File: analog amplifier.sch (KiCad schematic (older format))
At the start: 9 parts, among them U1 AD812

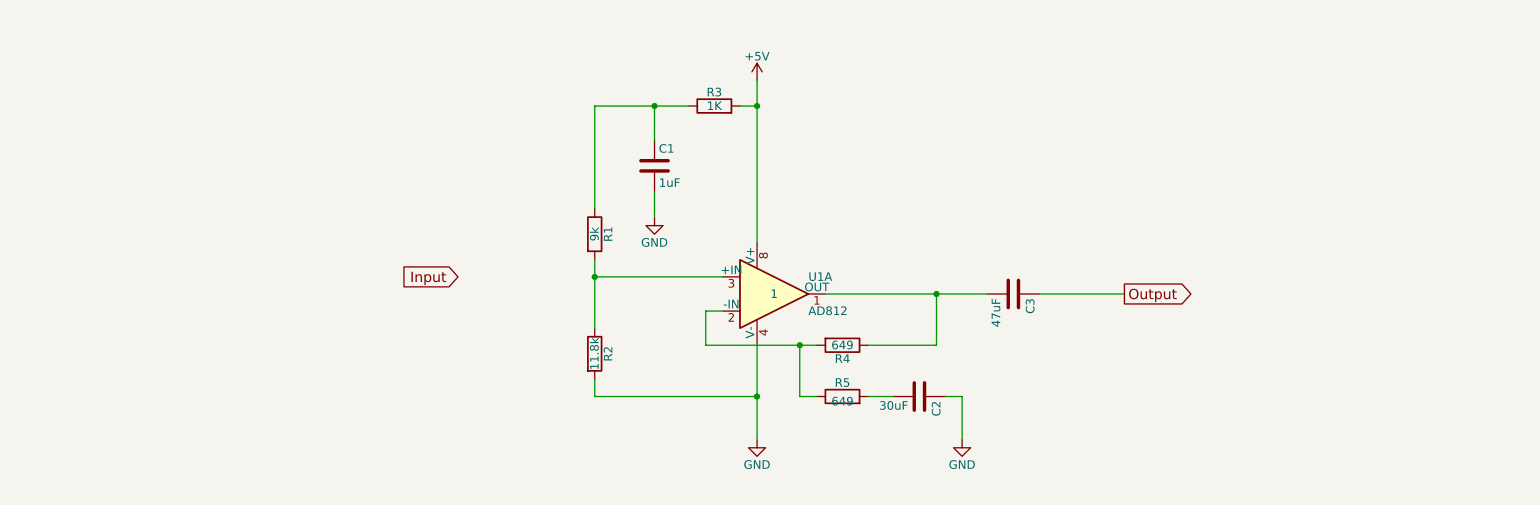
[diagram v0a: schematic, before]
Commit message: Add files via upload
Schematics and BOM
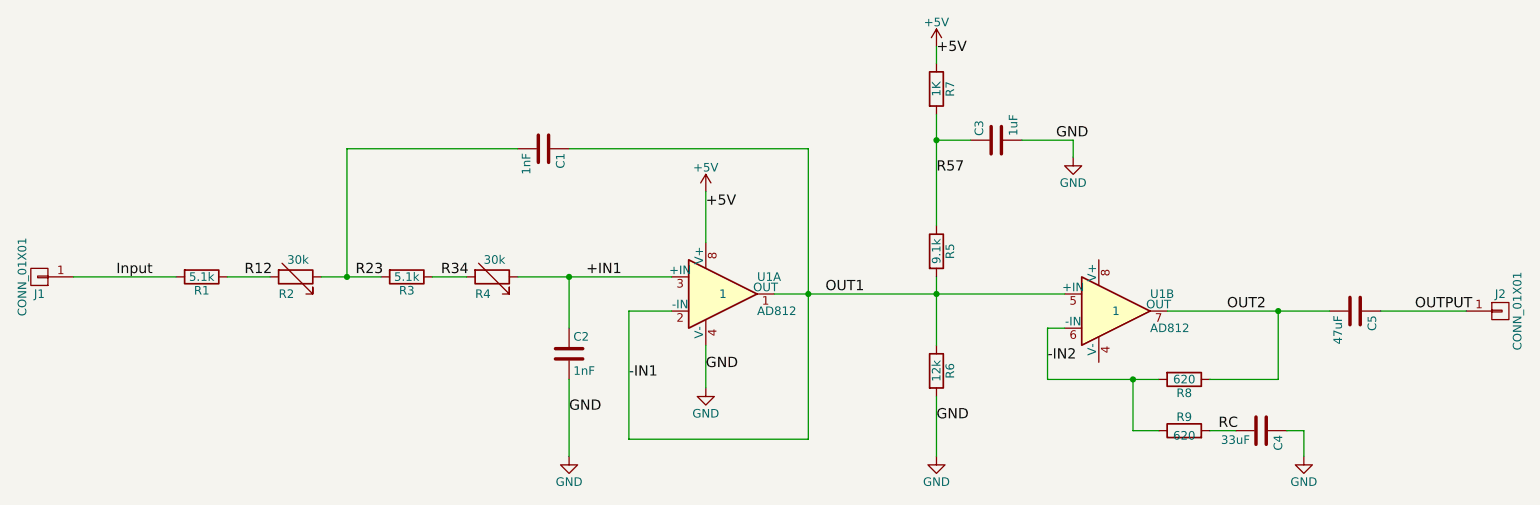
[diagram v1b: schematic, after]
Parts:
- added C1, C2: 1nF, Capacitors_SMD:C_0402, symbol C
- added J1, J2: CONN_01X01, Connectors:Banana_Jack_1Pin, symbol CONN_01X01
- added R1, R3: 5.1k, Resistors_SMD:R_0402, symbol R
- added R2, R4: 30k, Resistors_SMD:R_2816, symbol R_Variable
- added unit 1 of U1
- C3: renamed from C1; footprint (none) -> Capacitors_SMD:C_0603
- C4: renamed from C2; value 30uF -> 33uF; footprint (none) -> Capacitors_SMD:C_0805
- C5: renamed from C3; footprint (none) -> Capacitors_SMD:C_0805
- R5: renamed from R1; value 9k -> 9.1k; footprint (none) -> Resistors_SMD:R_0402
- R6: renamed from R2; value 11.8k -> 12k; footprint (none) -> Resistors_SMD:R_0402
- R7: renamed from R3; footprint (none) -> Resistors_SMD:R_0402
- R8: renamed from R4; value 649 -> 620; footprint (none) -> Resistors_SMD:R_0402
- R9: renamed from R5; value 649 -> 620; footprint (none) -> Resistors_SMD:R_0402
- U1: footprint (none) -> SMD_Packages:SOIC-8-N
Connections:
- net +5V: now also R7.1, U1.8 (V+); no longer R7.2, U1.8 (V+)
- net GND: now also C2.2, U1.4 (V-); no longer U1.4 (V-)
- net Input: now also J1.1 (P1), R1.2
- net OUT2: now reaches C5.2, R8.1
- net OUT2: now also U1.7 (OUT); no longer U1.1 (OUT)
- net -IN2: now reaches R8.2, R9.1
- net -IN2: now also U1.6 (-IN); no longer U1.2 (-IN)
- net -IN1: now reaches R5.2, R6.1
- net -IN1: now also U1.5 (+IN), C1.1, U1.1 (OUT), U1.2 (-IN); no longer U1.3 (+IN)
- net R57: now reaches C3.1, R5.1
- net R57: now also R7.2; no longer R7.1
- net RC: now reaches C4.2, R9.2
- net Output renamed OUTPUT
- net OUTPUT: now also J2.1 (P1)
- new net +IN1: C2.1, R4.1, U1.3 (+IN)
- new net R12: R1.1, R2.2
- new net R23: C1.2, R2.1, R3.2
- new net R34: R3.1, R4.2
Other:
- moved on the sheet: C3, C4, C5, R5, R6, R7, R8, R9
